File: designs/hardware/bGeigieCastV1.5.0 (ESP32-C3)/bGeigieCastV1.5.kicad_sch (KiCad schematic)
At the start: 10 parts, among them SW1 TACT-SWITCH, SW2 SWITCH_INV, U1 ESP32S, U2 XBEE-socket, U3 WeMos_D1_mini

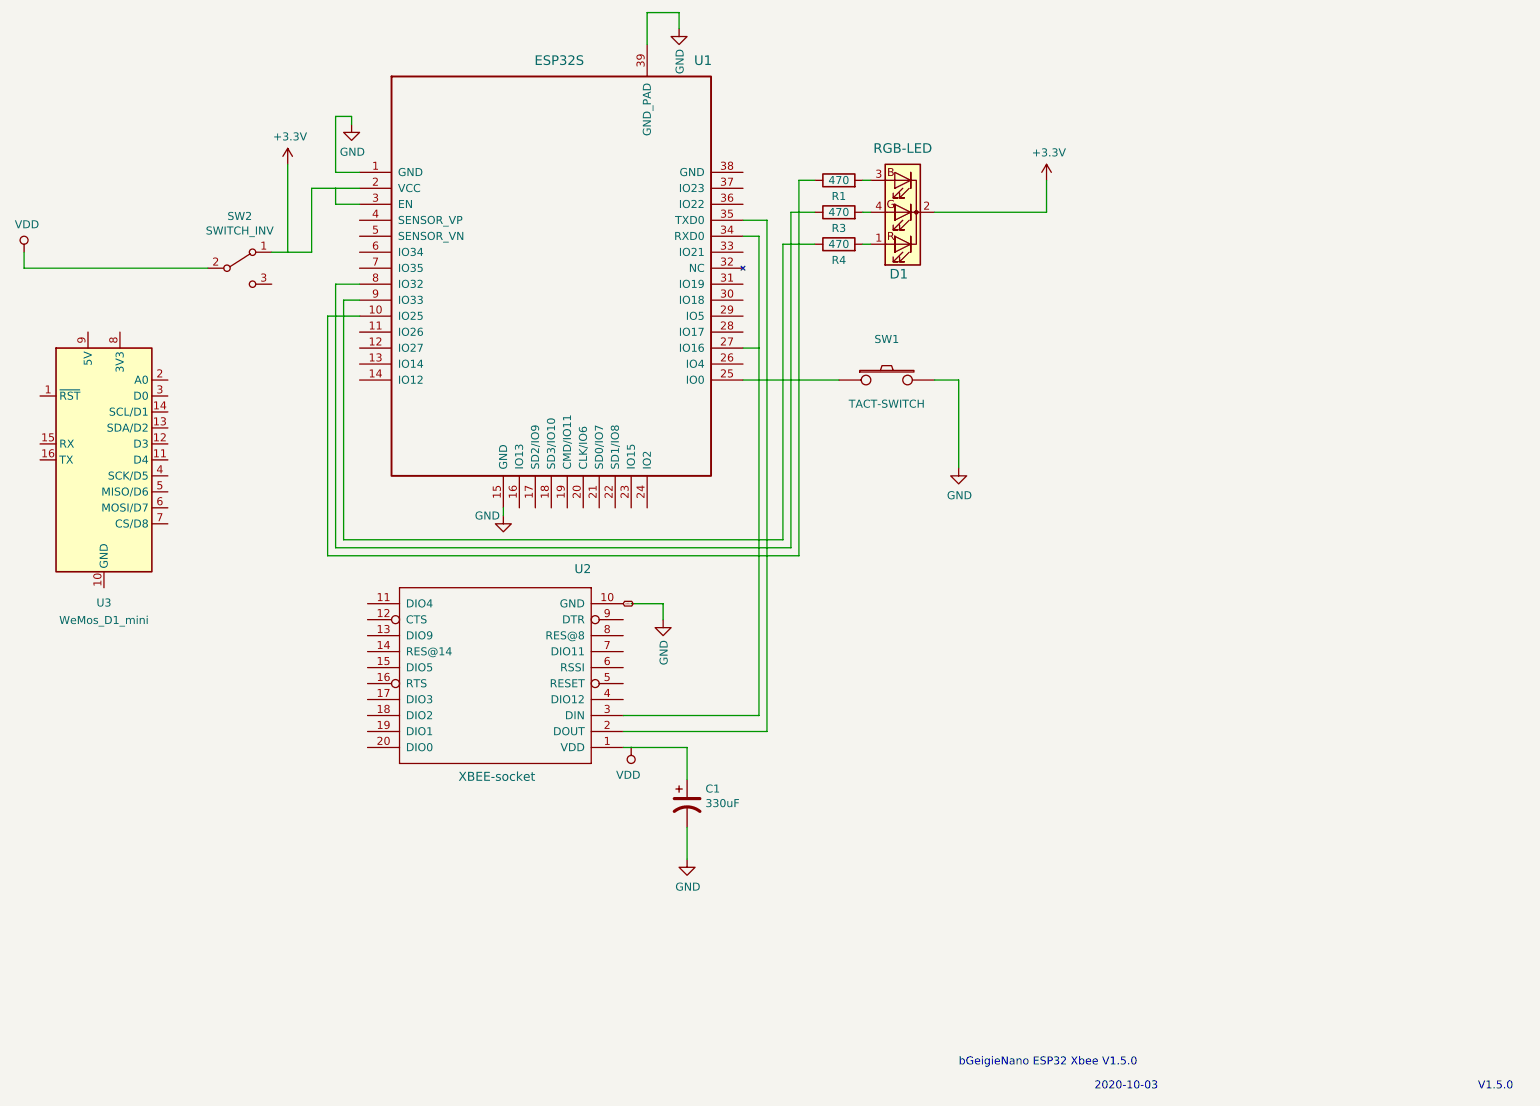
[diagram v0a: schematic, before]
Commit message: Update
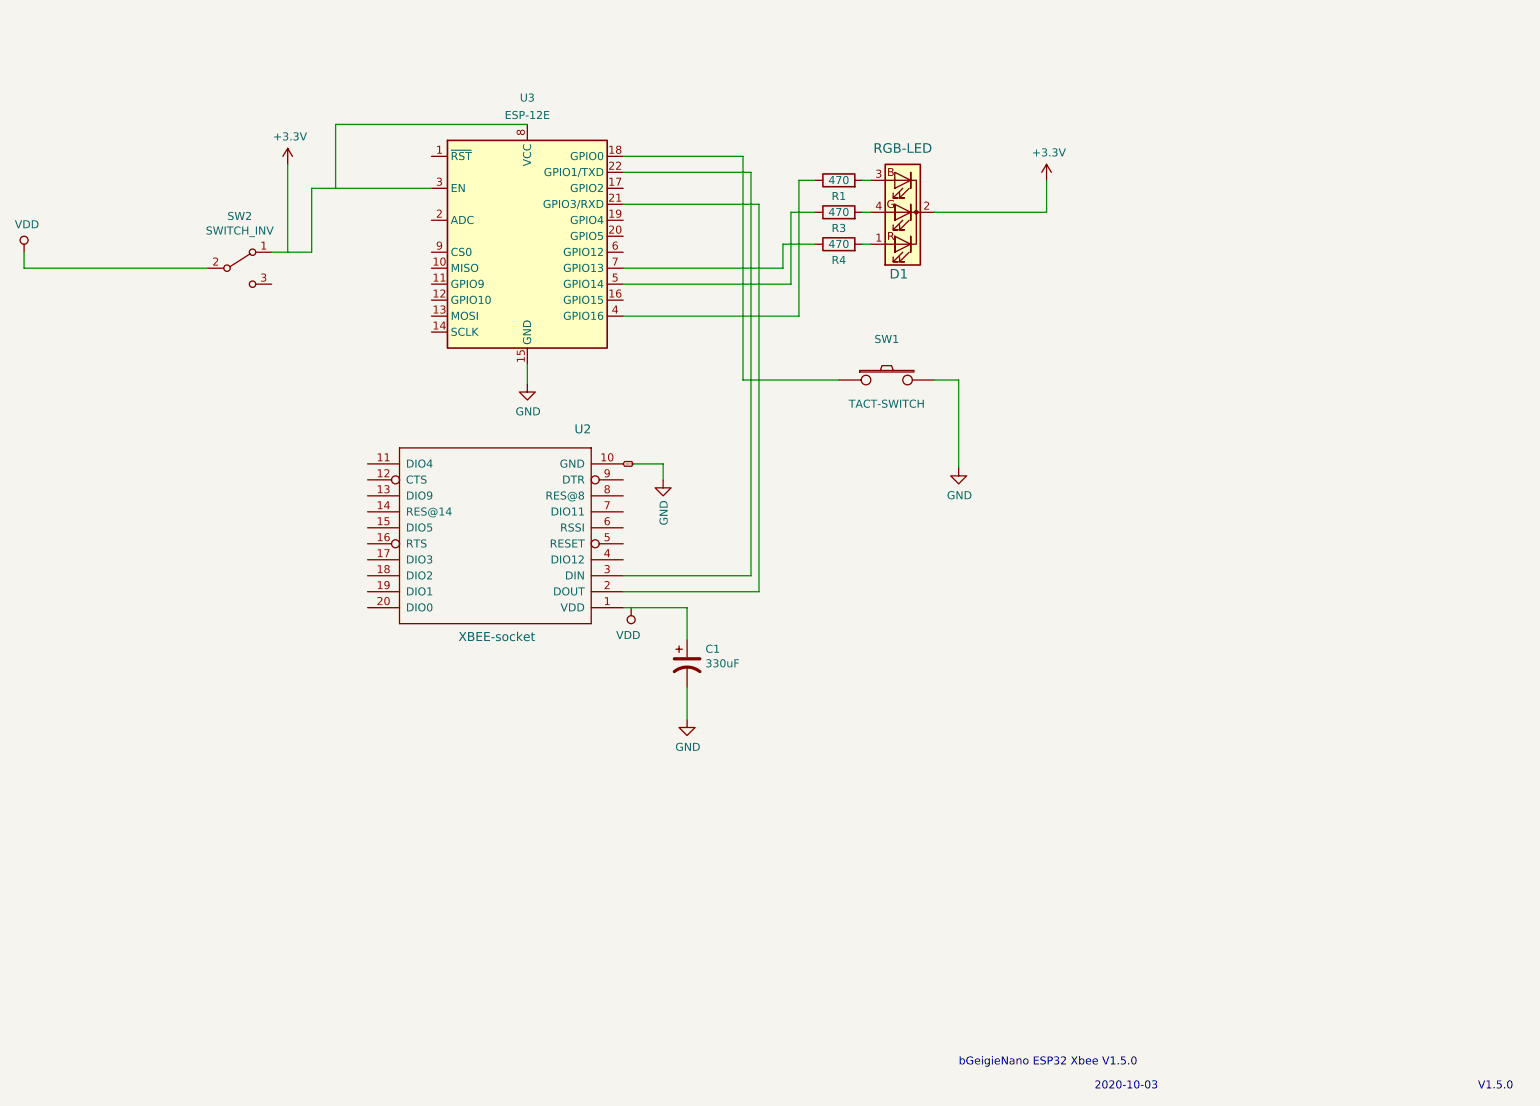
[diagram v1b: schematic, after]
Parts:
- removed U1: ESP32S, ESP32-footprints-Lib:ESP-32S, symbol xbee-rescue:ESP32S-espressif-xess
- removed U3: WeMos_D1_mini, RF_Module:ESP-12E, symbol MCU_Module:WeMos_D1_mini
- added U3: ESP-12E, RF_Module:ESP-12E, symbol RF_Module:ESP-12E
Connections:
- net +3V3: now also U3.3 (EN), U3.8 (VCC)
- net GND: now also U3.15 (GND)
- net at U2.2 (DOUT): now also U3.21 (GPIO3/RXD)
- net at U2.3 (DIN): now also U3.22 (GPIO1/TXD)
- net at SW1.1: now also U3.18 (GPIO0)
- net at R1.1: now also U3.4 (GPIO16)
- net at R3.1: now also U3.5 (GPIO14)
- net at R4.1: now also U3.7 (GPIO13)
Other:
- moved on the sheet: C1, U2
